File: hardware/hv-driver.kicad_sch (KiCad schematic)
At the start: 6 parts, among them IC2 CD4504BM, U4 HV5622PG

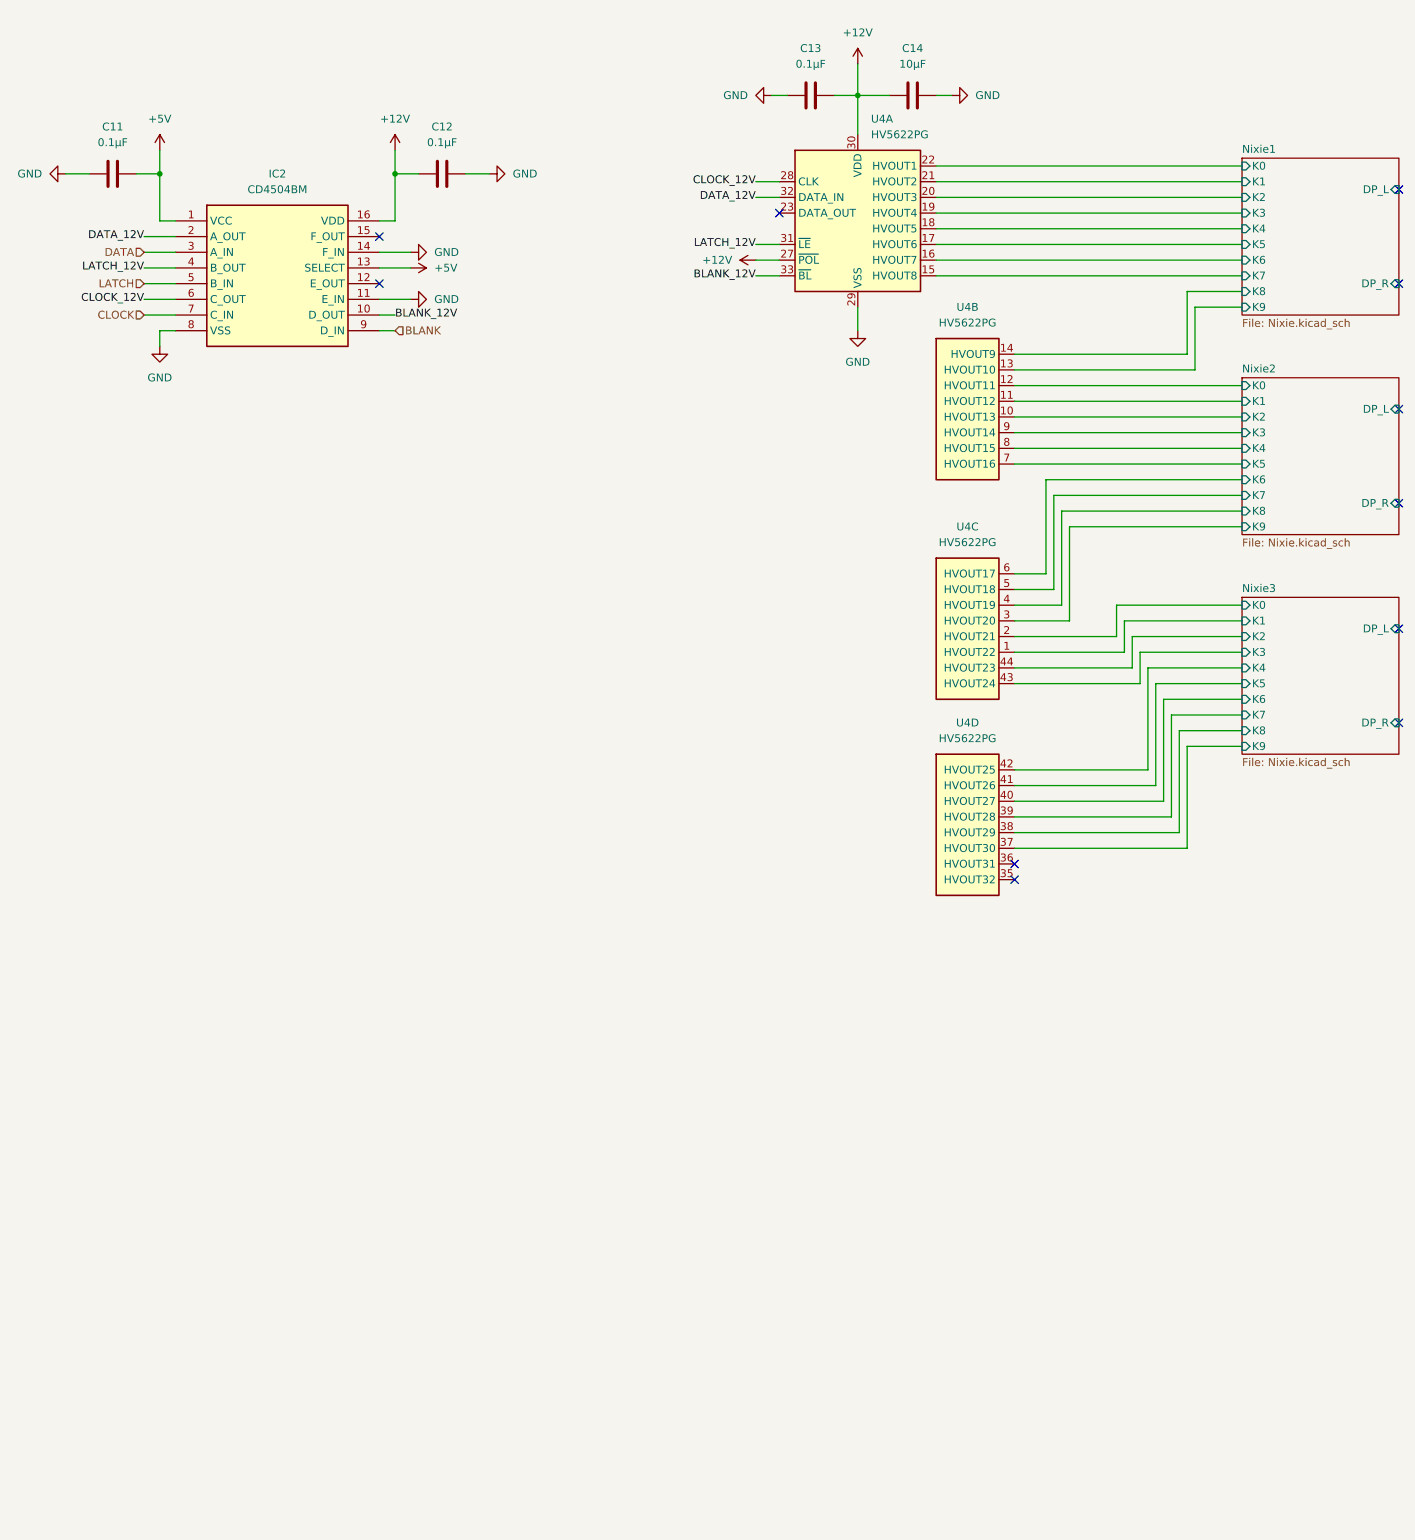
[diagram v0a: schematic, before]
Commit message: WIP SN74141 redesign
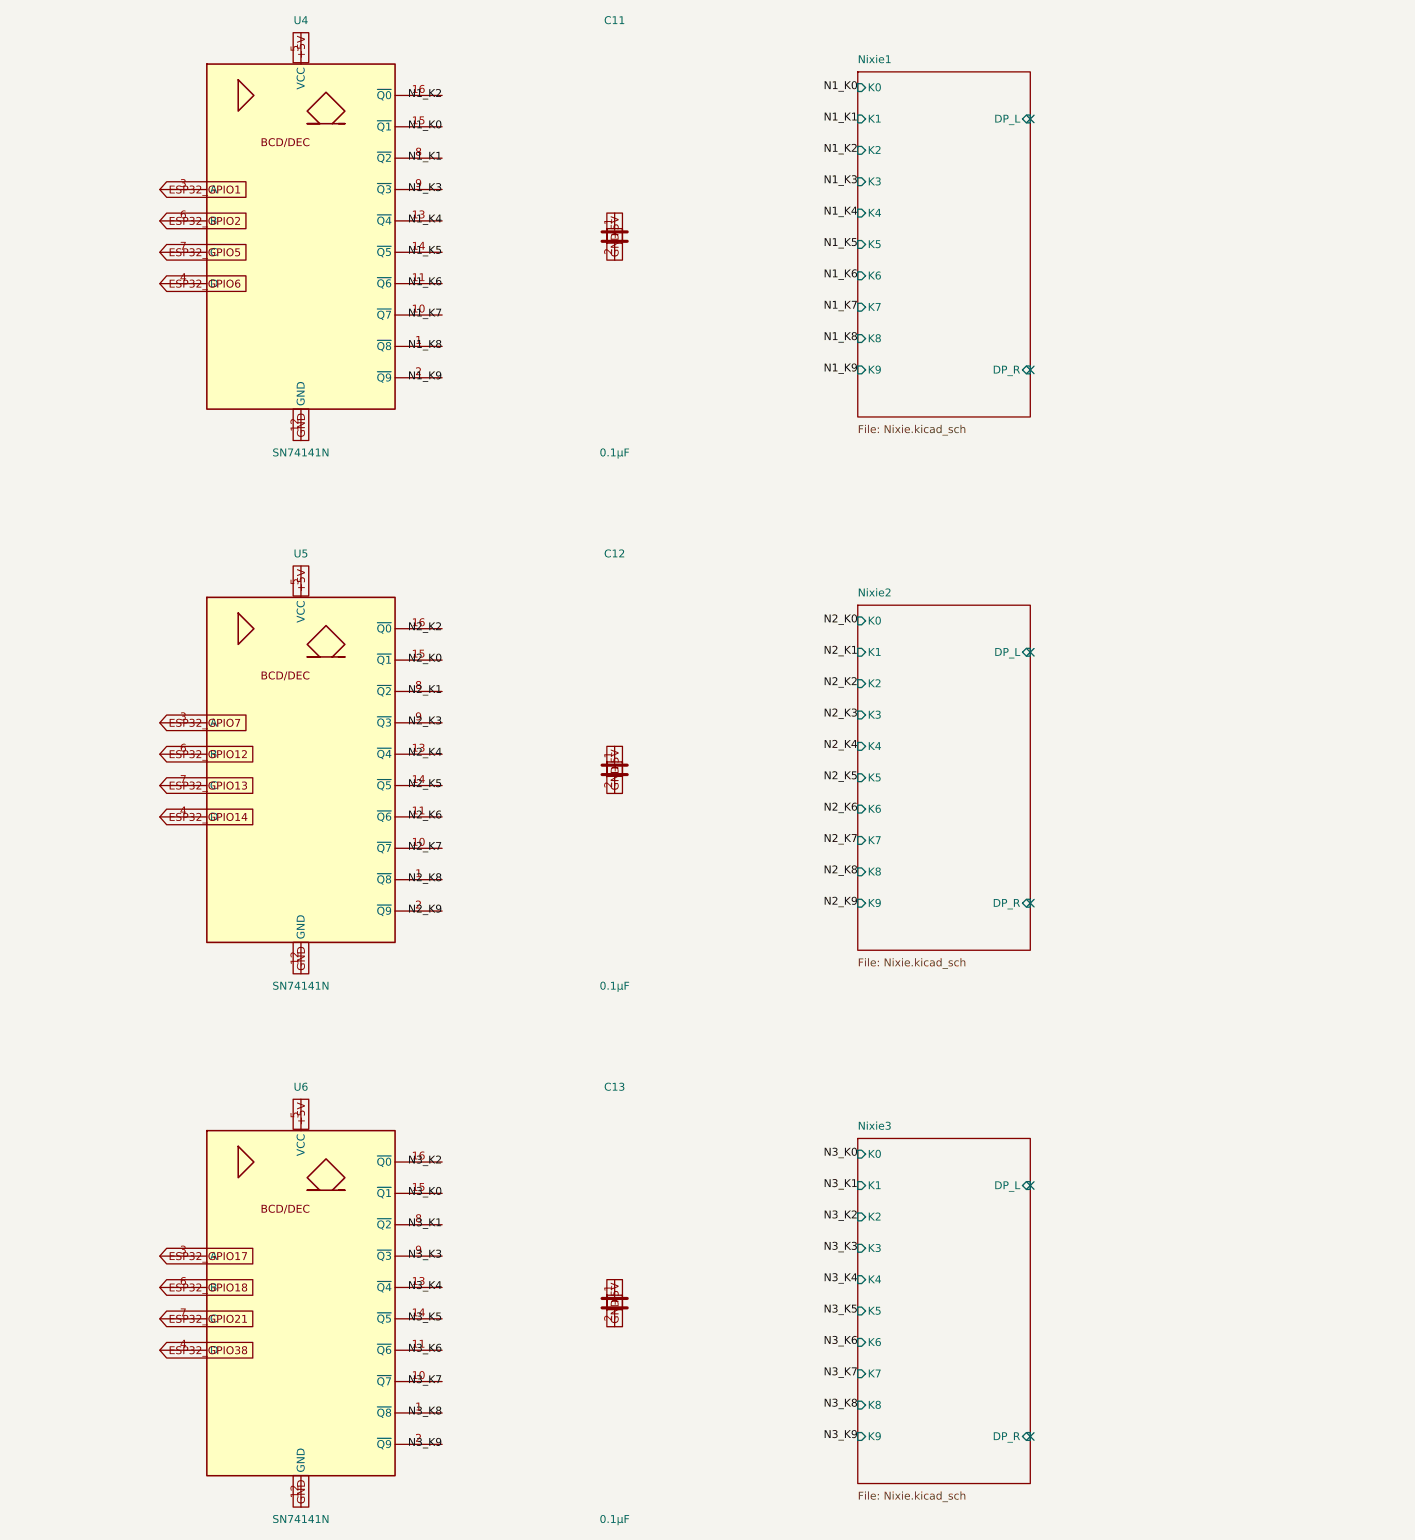
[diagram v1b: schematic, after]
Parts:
- removed C14: 10µF, Capacitor_SMD:C_1206_3216Metric, symbol Device:C
- removed IC2: CD4504BM, nixie-esp32:SOIC127P600X175-16N, symbol nixie-esp32:CD4504BM
- removed U4: HV5622PG, Package_QFP:PQFP-44_10x10mm_P0.8mm, symbol Driver_Display:HV5622PG
- added U4, U5, U6: SN74141N, Package_DIP:DIP-16_W7.62mm, symbol 74xx_IEEE:74141
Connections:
- net +5V: now also C12.1, C13.1, U4.5 (VCC), U5.5 (VCC), U6.5 (VCC)
- net GND: now also C13.2, U4.12 (GND), U5.12 (GND), U6.12 (GND); no longer C13.1
- removed net +12V: C12.1, C13.2
- new net ESP32_GPIO1: U4.3 (A)
- new net ESP32_GPIO12: U5.6 (B)
- new net ESP32_GPIO13: U5.7 (C)
- new net ESP32_GPIO14: U5.4 (D)
- new net ESP32_GPIO17: U6.3 (A)
- new net ESP32_GPIO18: U6.6 (B)
- new net ESP32_GPIO2: U4.6 (B)
- new net ESP32_GPIO21: U6.7 (C)
- new net ESP32_GPIO38: U6.4 (D)
- new net ESP32_GPIO5: U4.7 (C)
- new net ESP32_GPIO6: U4.4 (D)
- new net ESP32_GPIO7: U5.3 (A)
- new net N1_K0: U4.15 (~{Q1})
- new net N1_K1: U4.8 (~{Q2})
- new net N1_K2: U4.16 (~{Q0})
- new net N1_K3: U4.9 (~{Q3})
- new net N1_K4: U4.13 (~{Q4})
- new net N1_K5: U4.14 (~{Q5})
- new net N1_K6: U4.11 (~{Q6})
- new net N1_K7: U4.10 (~{Q7})
- new net N1_K8: U4.1 (~{Q8})
- new net N1_K9: U4.2 (~{Q9})
- new net N2_K0: U5.15 (~{Q1})
- new net N2_K1: U5.8 (~{Q2})
- new net N2_K2: U5.16 (~{Q0})
- new net N2_K3: U5.9 (~{Q3})
- new net N2_K4: U5.13 (~{Q4})
- new net N2_K5: U5.14 (~{Q5})
- new net N2_K6: U5.11 (~{Q6})
- new net N2_K7: U5.10 (~{Q7})
- new net N2_K8: U5.1 (~{Q8})
- new net N2_K9: U5.2 (~{Q9})
- new net N3_K0: U6.15 (~{Q1})
- new net N3_K1: U6.8 (~{Q2})
- new net N3_K2: U6.16 (~{Q0})
- new net N3_K3: U6.9 (~{Q3})
- new net N3_K4: U6.13 (~{Q4})
- new net N3_K5: U6.14 (~{Q5})
- new net N3_K6: U6.11 (~{Q6})
- new net N3_K7: U6.10 (~{Q7})
- new net N3_K8: U6.1 (~{Q8})
- new net N3_K9: U6.2 (~{Q9})
- no-connect marks 11 -> 6

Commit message: Resolve all DRC warnings
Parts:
- U4, U6: footprint Package_DIP:DIP-16_W7.62mm -> nixie-esp32:DIP-16_W7.62mm
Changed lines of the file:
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@@
     (property "Reference" "U4" (at 80.01 17.07 0))
     (property "Value" "SN74141N" (at 80.01 87.07 0))
-    (property "Footprint" "Package_DIP:DIP-16_W7.62mm" (at 80.01 52.07 0)
+    (property "Footprint" "nixie-esp32:DIP-16_W7.62mm" (at 80.01 52.07 0)
       (effects (font (size 1 1)) hide)
     )
@@
     (property "Reference" "U6" (at 80.01 189.79 0))
     (property "Value" "SN74141N" (at 80.01 259.78999999999996 0))
-    (property "Footprint" "Package_DIP:DIP-16_W7.62mm" (at 80.01 224.79 0)
+    (property "Footprint" "nixie-esp32:DIP-16_W7.62mm" (at 80.01 224.79 0)
       (effects (font (size 1 1)) hide)
     )
